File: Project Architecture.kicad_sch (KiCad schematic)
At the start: 0 parts

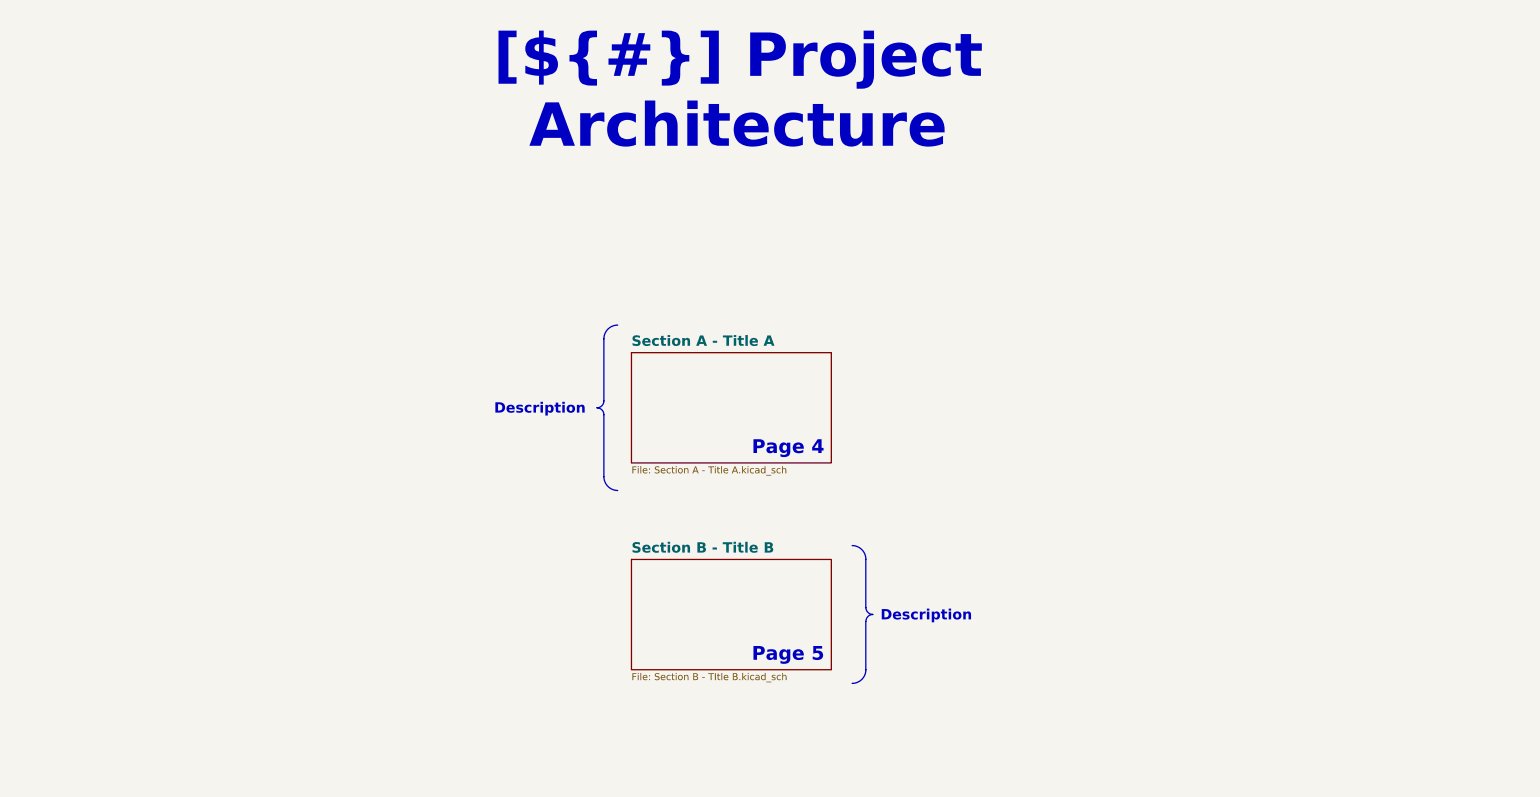
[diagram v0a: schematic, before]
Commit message: Frist draft of Schematic
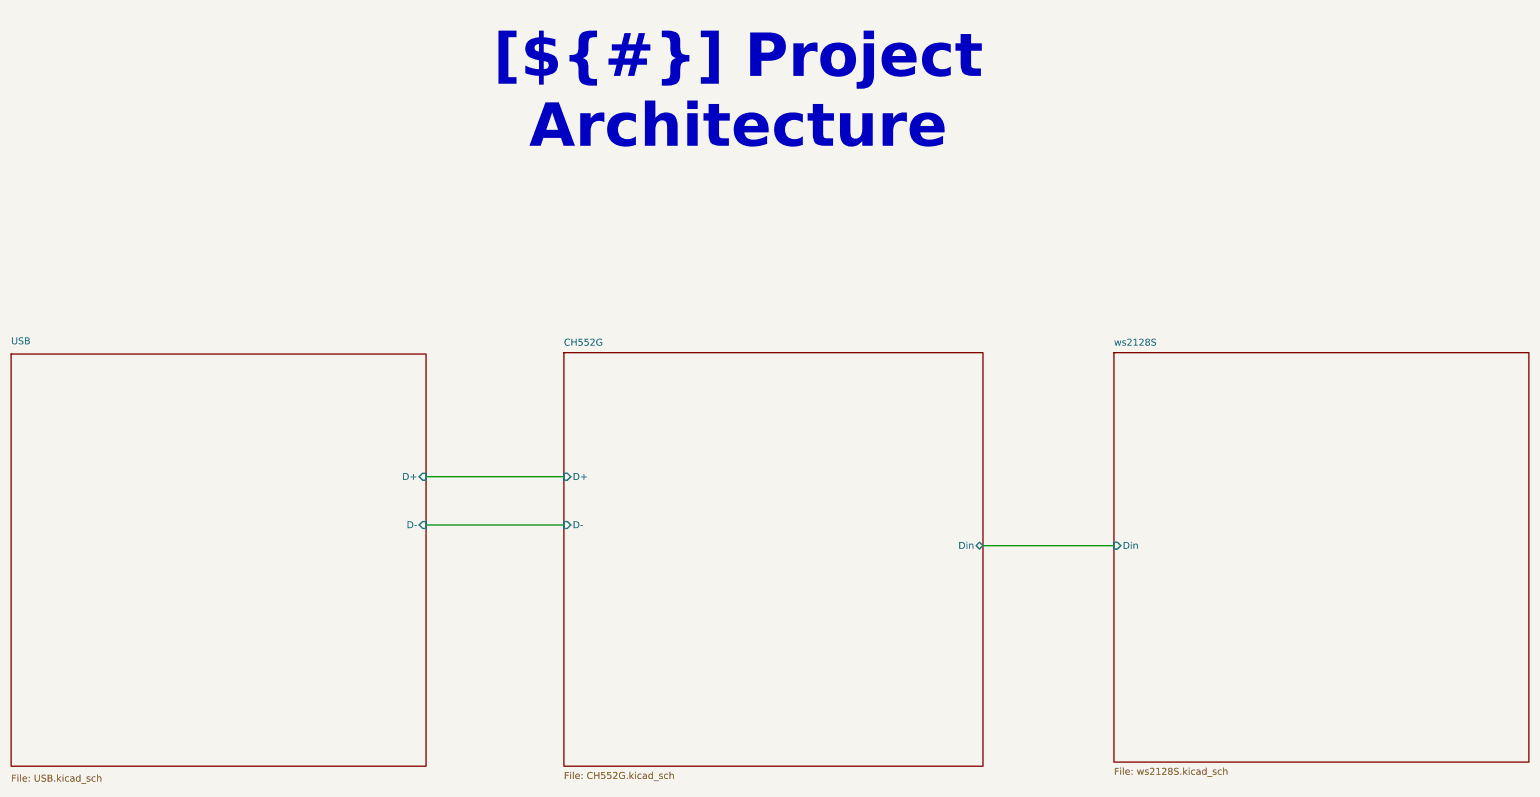
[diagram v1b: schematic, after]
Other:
- removed sheet Section A - Title A
- removed sheet Section B - Title B
- added sheet CH552G (CH552G.kicad_sch)
- added sheet USB (USB.kicad_sch)
- added sheet ws2128S (ws2128S.kicad_sch)
- note removed: "Page 4"
- note removed: "Page 5"
